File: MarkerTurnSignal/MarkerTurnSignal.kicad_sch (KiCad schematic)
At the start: 1 part, among them J0 C-

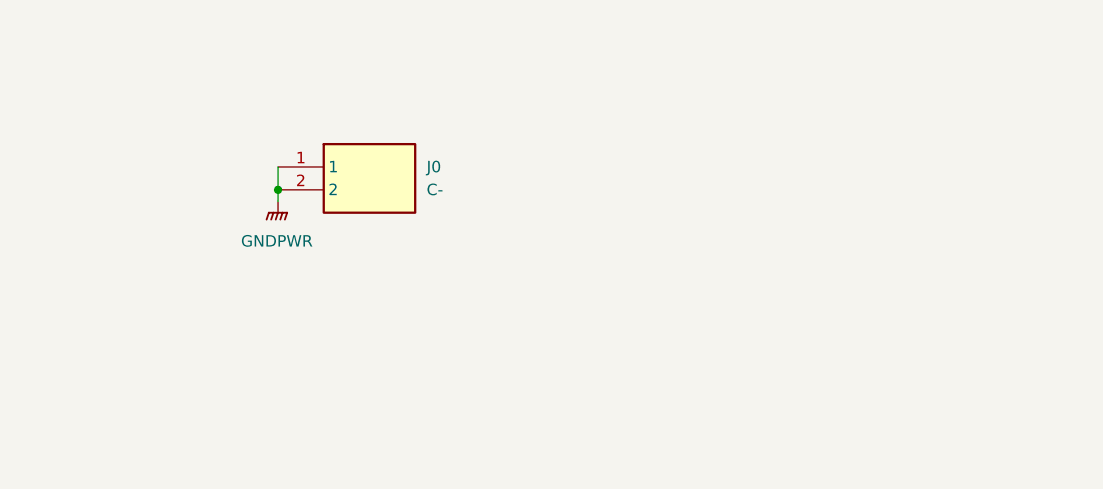
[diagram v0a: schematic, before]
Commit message: Completed light boards.
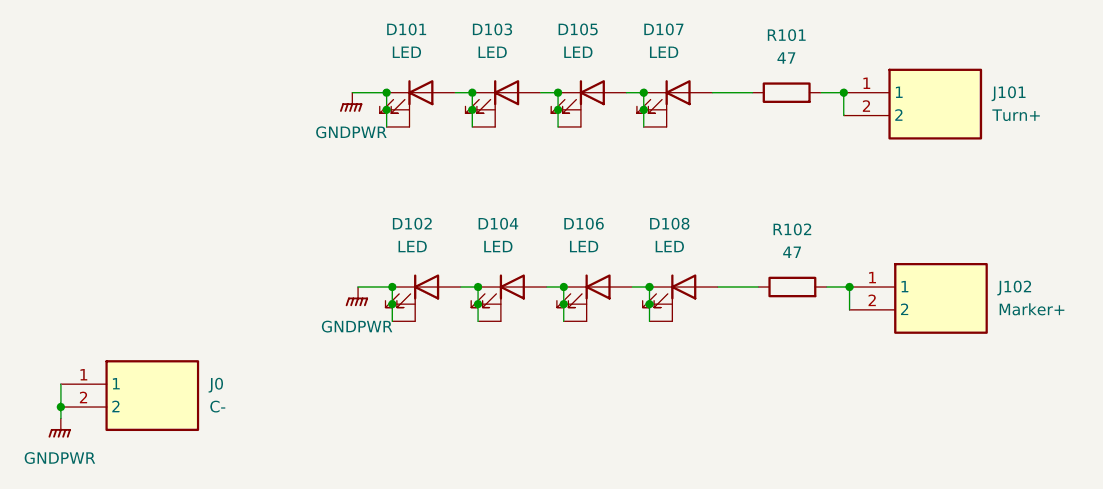
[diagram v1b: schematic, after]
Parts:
- added D101, D102, D103, D104, D105, D106, D107, D108: LED, LED_SMD:LED_Avago_PLCC4_3.2x2.8mm_CW, symbol Device:LED
- added J101: Turn+, SpadeLugs:197054303, symbol SpadeLugs:19705-4303
- added J102: Marker+, SpadeLugs:197054303, symbol SpadeLugs:19705-4303
- added R101, R102: 47, Resistor_SMD:R_0603_1608Metric, symbol Device:R
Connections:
- net GNDPWR: now also D101.1 (K), D101.3 (K), D101.4 (K), D102.1 (K), D102.3 (K), D102.4 (K)
- new net: D107.2 (A), R101.1
- new net: J101.1, J101.2, R101.2
- new net: D101.2 (A), D103.1 (K), D103.3 (K), D103.4 (K)
- new net: D103.2 (A), D105.1 (K), D105.3 (K), D105.4 (K)
- new net: D105.2 (A), D107.1 (K), D107.3 (K), D107.4 (K)
- new net: D106.2 (A), D108.1 (K), D108.3 (K), D108.4 (K)
- new net: D108.2 (A), R102.1
- new net: D104.2 (A), D106.1 (K), D106.3 (K), D106.4 (K)
- new net: J102.1, J102.2, R102.2
- new net: D102.2 (A), D104.1 (K), D104.3 (K), D104.4 (K)
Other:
- moved on the sheet: J0
